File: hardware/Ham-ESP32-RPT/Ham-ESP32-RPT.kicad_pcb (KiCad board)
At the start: 2 copper layers, 100 x 115 mm, 9 parts, among them J5 Conn_01x04_Socket, Q1 MMBT3904, SW1 REP TEST, U4 ESP32-S3-DevKitC

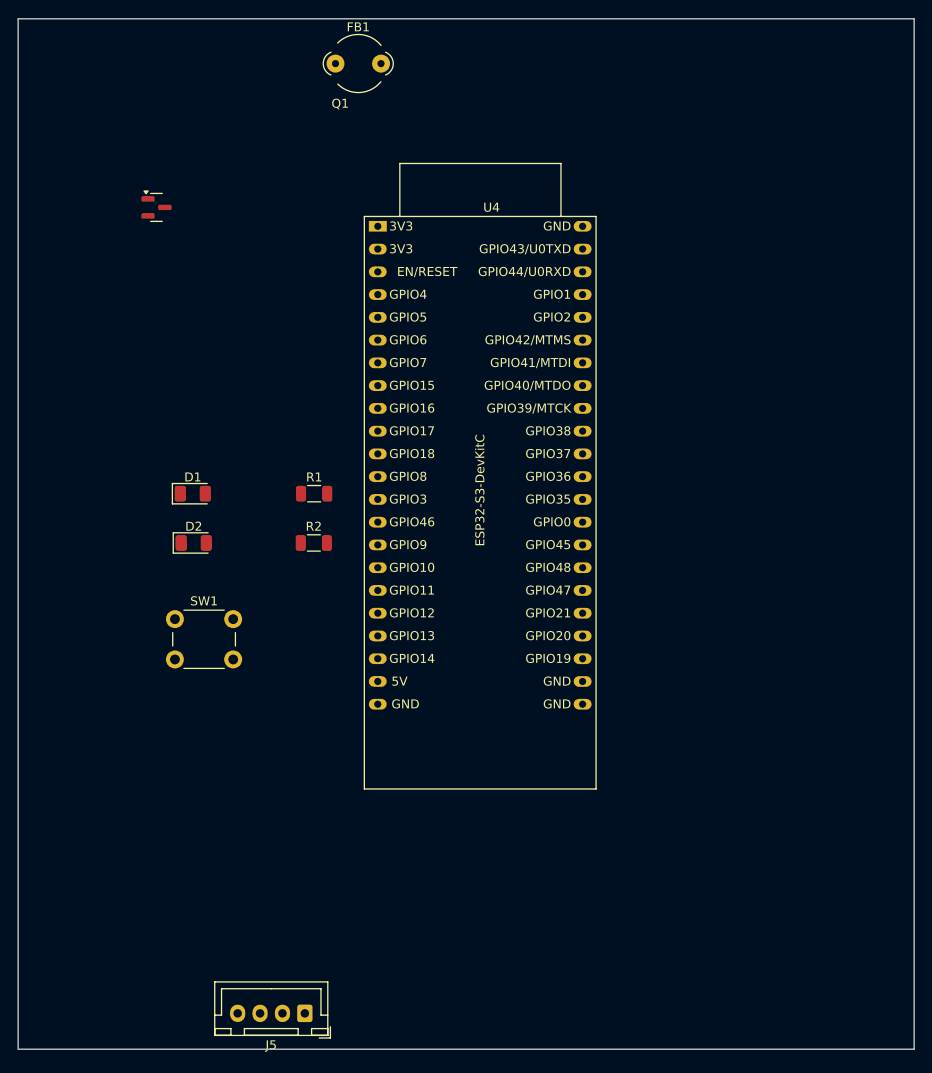
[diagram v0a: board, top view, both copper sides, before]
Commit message: PCB kicad update
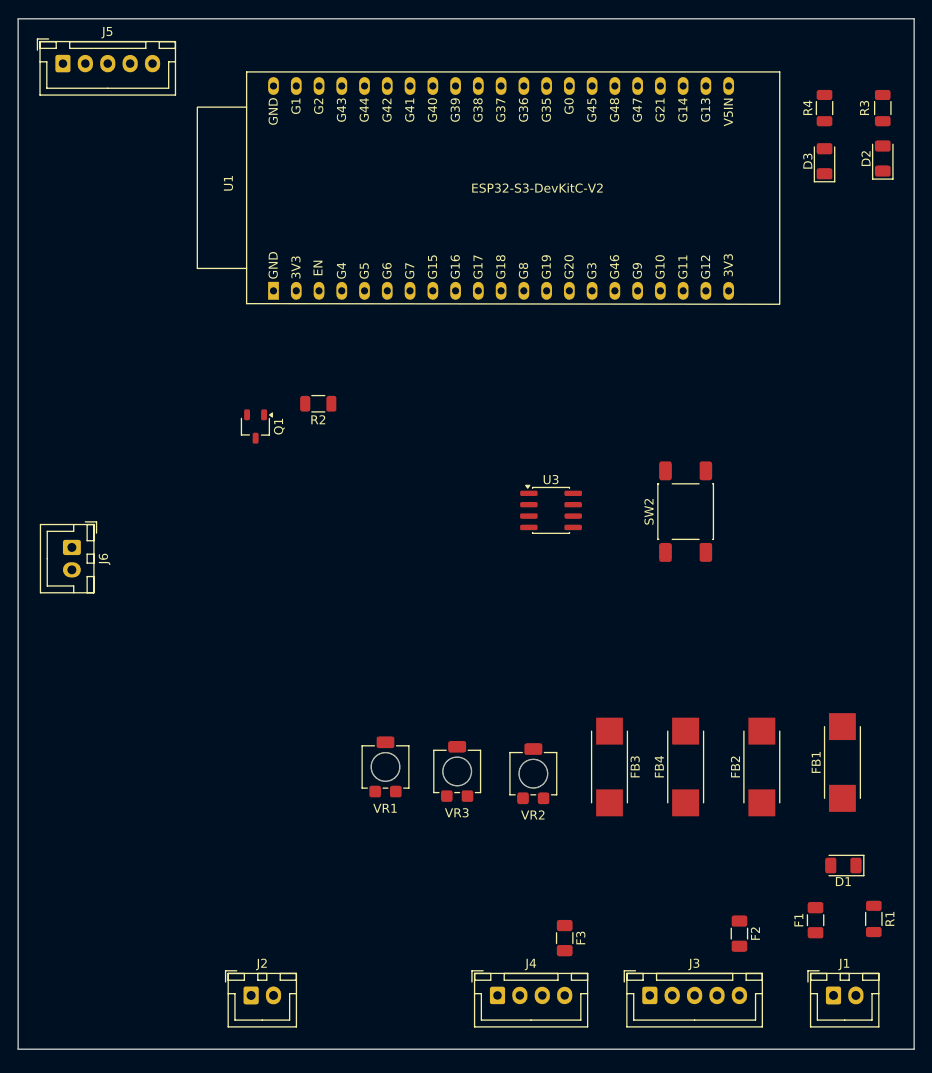
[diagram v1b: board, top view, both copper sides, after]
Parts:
- removed SW1: REP TEST, Button_Switch_THT:SW_PUSH_6mm
- removed U4: ESP32-S3-DevKitC, PCM_Espressif:ESP32-S3-DevKitC
- added D3: GREEN, LED_SMD:LED_1206_3216Metric, F.Cu at (161.5, 54.9)
- added F1: 2A, Fuse:Fuse_1206_3216Metric, F.Cu at (160.5, 139.6)
- added F2: 4A, Fuse:Fuse_1206_3216Metric, F.Cu at (152.0, 141.1)
- added F3: 4A, Fuse:Fuse_1206_3216Metric, F.Cu at (132.5, 141.6)
- added FB2: VK200, Inductor_SMD:L_Neosid_MicroCoil_Ms36-L, F.Cu at (154.5, 122.5)
- added FB3: VK200, Inductor_SMD:L_Neosid_MicroCoil_Ms36-L, F.Cu at (137.5, 122.5)
- added FB4: VK200, Inductor_SMD:L_Neosid_MicroCoil_Ms36-L, F.Cu at (146.0, 122.5)
- added J1: 5V SUPPLY, Connector_JST:JST_XH_B2B-XH-A_1x02_P2.50mm_Vertical, F.Cu at (162.5, 148.0)
- added J2: 12V SUPPLY, Connector_JST:JST_XH_B2B-XH-A_1x02_P2.50mm_Vertical, F.Cu at (97.5, 148.0)
- added J3: RX RADIO, Connector_JST:JST_XH_B5B-XH-A_1x05_P2.50mm_Vertical, F.Cu at (142.0, 148.0)
- added J4: TX RADIO, Connector_JST:JST_XH_B4B-XH-A_1x04_P2.50mm_Vertical, F.Cu at (125.0, 148.0)
- added J6: SPEAKER, Connector_JST:JST_XH_B2B-XH-A_1x02_P2.50mm_Vertical, F.Cu at (77.5, 98.0)
- added R3: 330R, Resistor_SMD:R_1206_3216Metric, F.Cu at (168.0, 49.0)
- added R4: 330R, Resistor_SMD:R_1206_3216Metric, F.Cu at (161.5, 49.0)
- added SW2: TEST, Button_Switch_SMD:SW_Push_1P1T_NO_E-Switch_TL3301NxxxxxG, F.Cu at (146.0, 94.0)
- added U1: ESP32-S3-DevKitC-V2, Ham-ESP32-RPT-pretty:ESP32-S3-DevKitC-V2, F.Cu at (100.0, 69.4)
- added U3: INA219AxD, Package_SO:SOIC-8_3.9x4.9mm_P1.27mm, F.Cu at (131.0, 93.9)
- added VR1: 10K, Potentiometer_SMD:Potentiometer_Bourns_3314R-1_Vertical_Hole, F.Cu at (112.5, 122.5)
- added VR2: 10K, Potentiometer_SMD:Potentiometer_Bourns_3314R-1_Vertical_Hole, F.Cu at (129.0, 123.2)
- added VR3: 10K, Potentiometer_SMD:Potentiometer_Bourns_3314R-1_Vertical_Hole, F.Cu at (120.5, 123.0)
- D1: value GREEN -> BLUE
- FB1: value FerriteBead -> VK200; footprint Ferrite_THT:LairdTech_28C0236-0JW-10 -> Inductor_SMD:L_Neosid_MicroCoil_Ms36-L
- J5: value Conn_01x04_Socket -> AUX BTN LED; footprint Connector_JST:JST_XH_B4B-XH-A_1x04_P2.50mm_Vertical -> Connector_JST:JST_XH_B5B-XH-A_1x05_P2.50mm_Vertical
- Q1: value MMBT3904 -> MMBT2222A; footprint Package_TO_SOT_SMD:SOT-23 -> Package_TO_SOT_SMD:TSOT-23
- R2: value 330R -> 3.3K
- moved J5 109.4 mm to (76.5, 44.0), turned to 0 degrees
- moved FB1 96.4 mm to (163.5, 122.0), turned to 90 degrees
- moved D2 88.1 mm to (168.0, 54.6), turned to 90 degrees
- moved D1 83.6 mm to (163.6, 133.5), turned to 180 degrees
- moved R1 78.4 mm to (167.0, 139.5), turned to -90 degrees
- moved Q1 26.8 mm to (98.0, 84.5), turned to -90 degrees
- moved R2 15.5 mm to (105.0, 82.0), turned to 180 degrees
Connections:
- D1 pad 1: GND -> Net-(D1-K)
- FB1 pad 1: unconnected-(FB1-Pad1) -> Net-(D1-A)
- FB1 pad 2: unconnected-(FB1-Pad2) -> +5V
- Q1 pad 1: unconnected-(Q1-B-Pad1) -> Net-(Q1-B)
- Q1 pad 2: unconnected-(Q1-E-Pad2) -> GND
- Q1 pad 3: unconnected-(Q1-C-Pad3) -> Net-(J4-Pin_1)
- R1 pad 1: Net-(U4-GPIO9/ADC1_CH8) -> Net-(D1-K)
- R1 pad 2: Net-(D1-A) -> GND
- R2 pad 2: Net-(D2-A) -> Net-(Q1-B)
